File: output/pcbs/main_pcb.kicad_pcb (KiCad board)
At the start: 2 copper layers, 147.5 x 112.7 mm, 78 parts

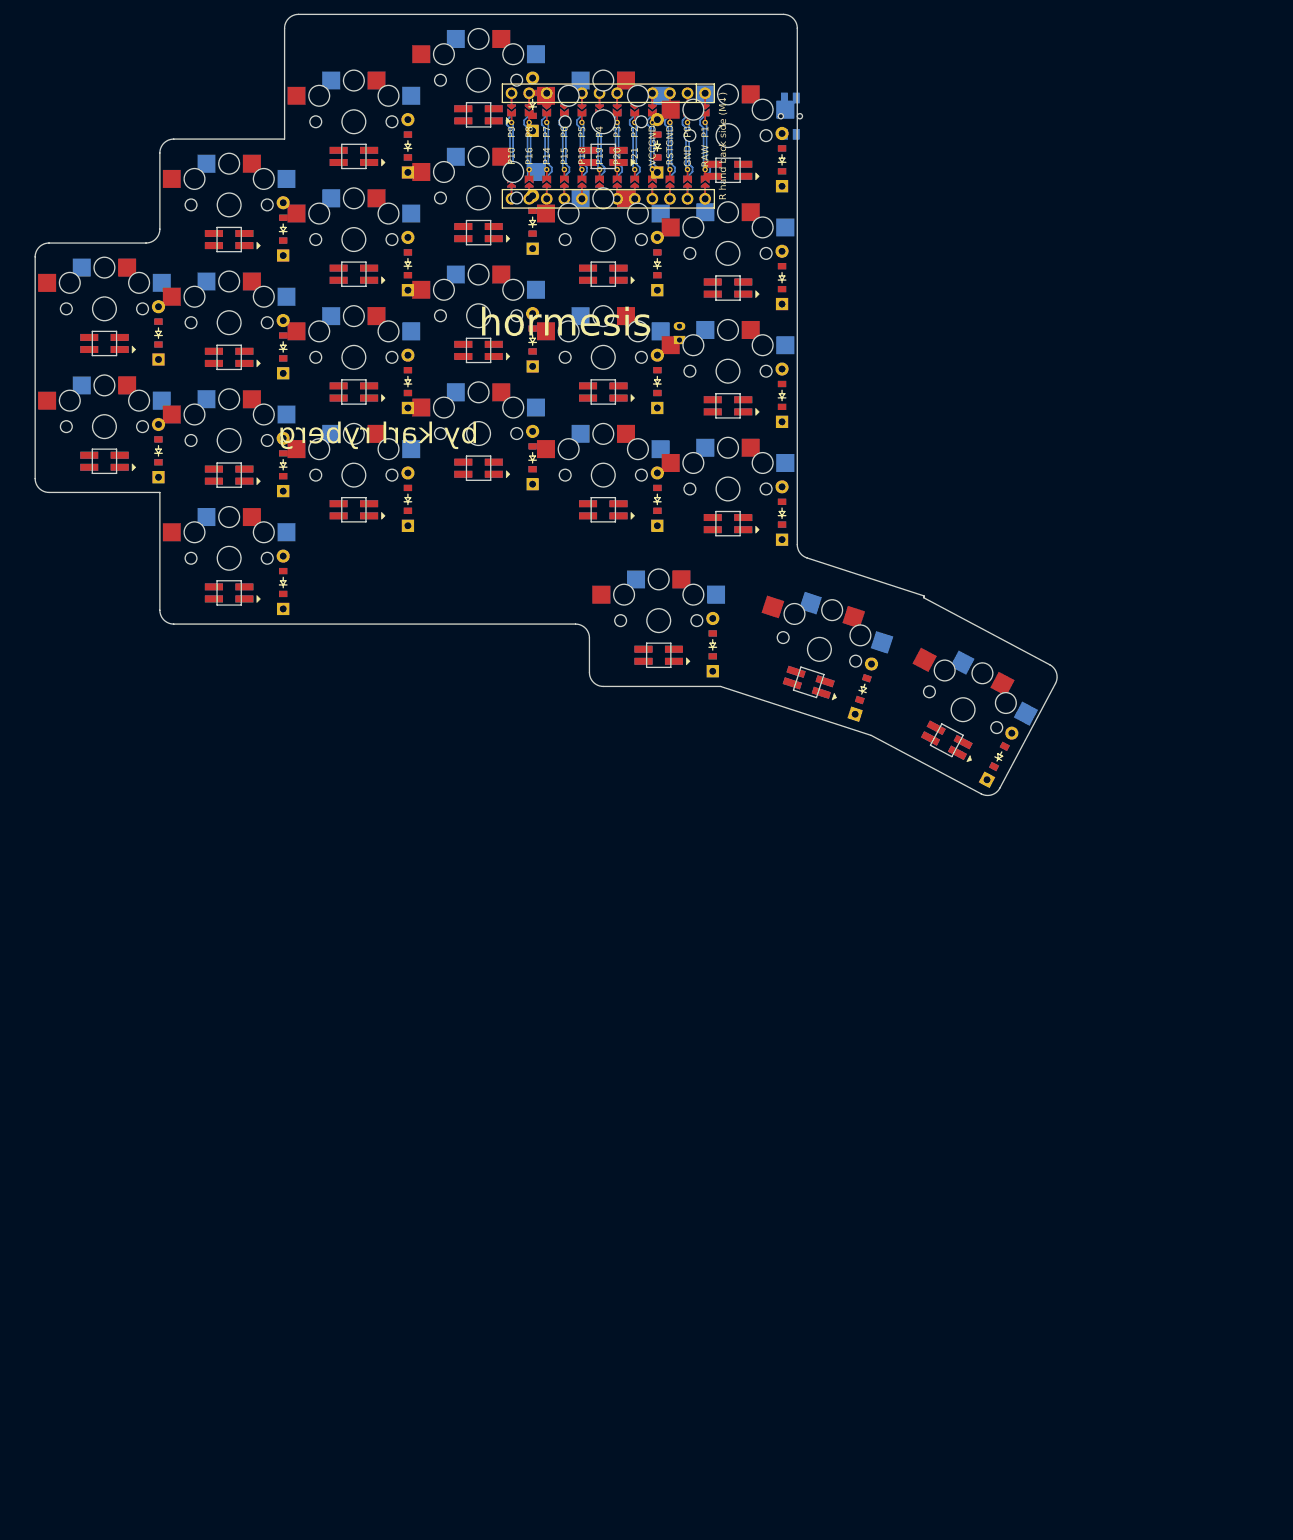
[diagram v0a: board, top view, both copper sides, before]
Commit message: Positions determined (more or less)
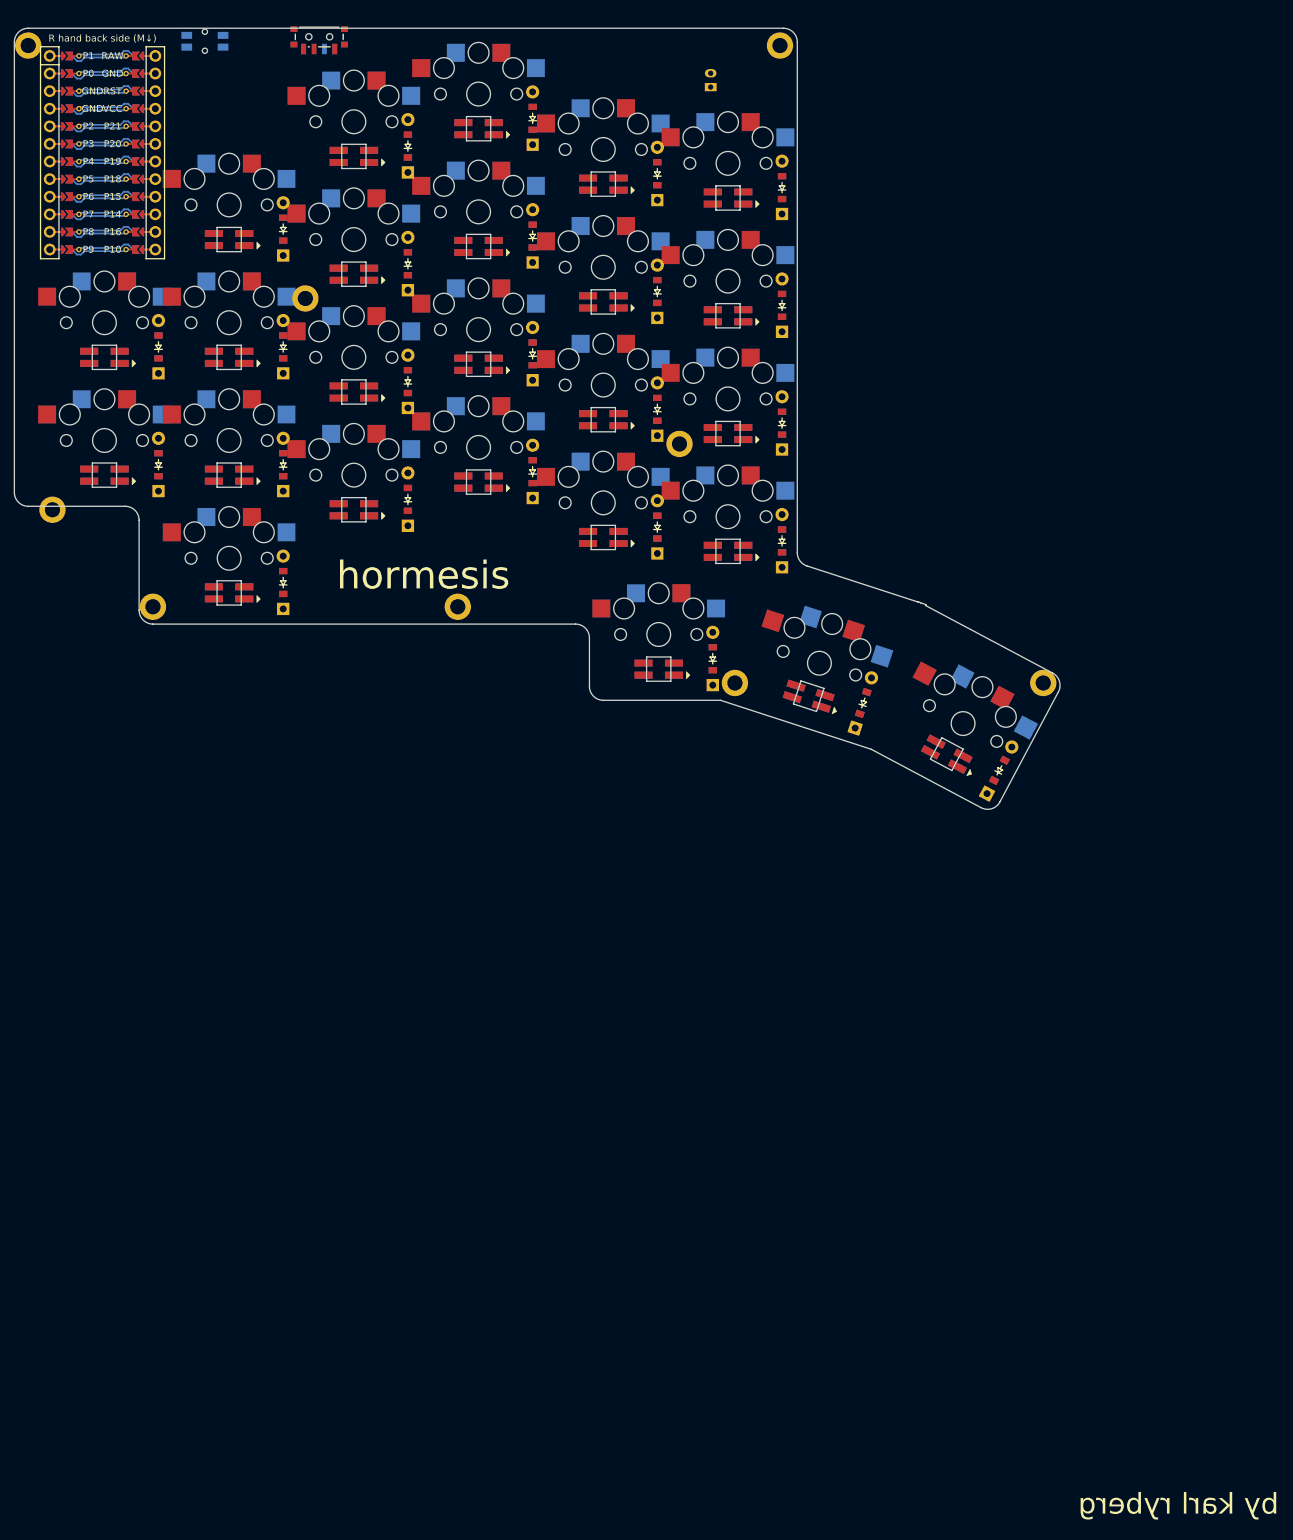
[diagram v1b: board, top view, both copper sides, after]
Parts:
- added H1: , mounting_hole, F.Cu at (217.5, 168.0)
- added H2: , mounting_hole, F.Cu at (179.5, 76.0)
- added H3: , mounting_hole, F.Cu at (89.0, 157.0)
- added H4: , mounting_hole, F.Cu at (74.5, 143.0)
- added H5: , mounting_hole, F.Cu at (173.0, 168.0)
- added H6: , mounting_hole, F.Cu at (133.0, 157.0)
- added H7: , mounting_hole, F.Cu at (111.0, 112.5)
- added H8: , mounting_hole, F.Cu at (165.0, 133.5)
- added H9: , mounting_hole, F.Cu at (71.0, 76.0)
- added SW1: , power_switch, F.Cu at (113.0, 74.8)
- moved B1 85.2 mm to (96.5, 75.4), turned to 0 degrees
- moved MCU1 74.3 mm to (81.7, 90.2), turned to 0 degrees
- moved JST1 36.8 mm to (169.5, 81.0)
- moved D13 4.00 mm to (161.8, 145.5)
- moved D14 4.00 mm to (161.8, 128.5)
- moved D15 4.00 mm to (161.8, 111.5)
- moved D16 4.00 mm to (161.8, 94.5)
- moved D17 4.00 mm to (179.8, 147.5)
- moved D18 4.00 mm to (179.8, 130.5)
- moved D19 4.00 mm to (179.8, 113.5)
- moved D20 4.00 mm to (179.8, 96.5)
- moved LED13 4.00 mm to (154.0, 147.0)
- moved LED14 4.00 mm to (154.0, 130.0)
- moved LED15 4.00 mm to (154.0, 113.0)
- moved LED16 4.00 mm to (154.0, 96.0)
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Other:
- board size 147.5 x 112.7 mm -> 150.9 x 112.7 mm
